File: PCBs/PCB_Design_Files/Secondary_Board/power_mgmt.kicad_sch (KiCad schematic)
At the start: 19 parts, among them Q3 MMBT3904, Q4 MMBT3904, U5 TPS61023DRLR, U6 TLV9101IDCKR

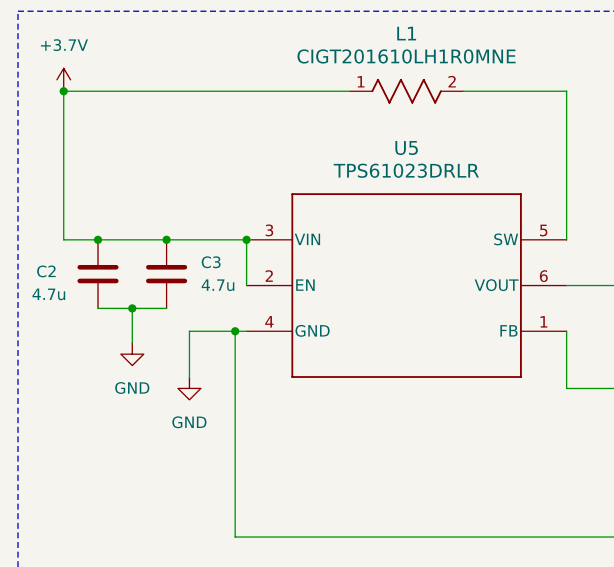
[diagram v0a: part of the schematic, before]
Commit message: updte
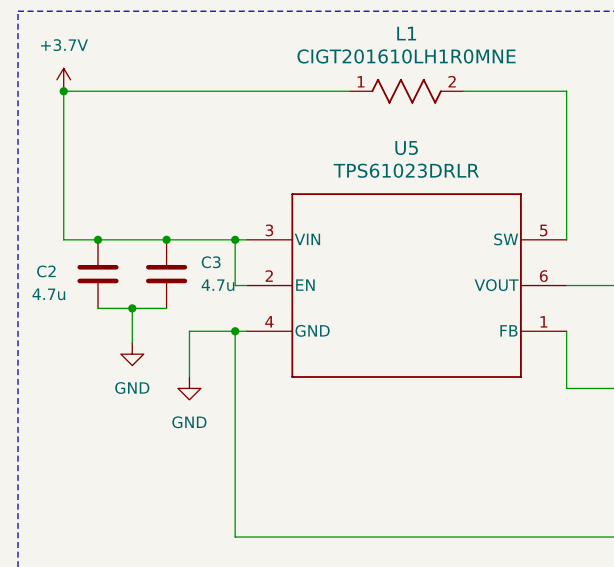
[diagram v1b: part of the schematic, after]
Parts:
- removed U5: TPS61023DRLR, Project Footprints:DRL0006A, symbol TPS61023:TPS61023DRLR
- added U5: TPS61023DRLR, Project Footprints:DRL0006A, symbol Project_Symbols:TPS61023DRLR
- BT1: footprint Diode_THT:D_DO-35_SOD27_P7.62mm_Horizontal -> Connector_JST:JST_PH_S2B-PH-K_1x02_P2.00mm_Horizontal
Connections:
- net +3.7V: now also U5.2 (EN), U5.3 (VIN)
- net +5V: now also U5.6 (VOUT)
- net GND: now also U5.4 (GND)
- net at R1.2, R2.1: now also U5.1 (FB)
- net at L1.2: now also U5.5 (SW)
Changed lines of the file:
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@@
+	)
+	(junction
+		(at 36.83 87.63)
+		(diameter 0)
+		(color 0 0 0 0)
 	)
 	(junction
@@
 	)
 	(junction
-		(at 36.83 87.63)
-		(diameter 0)
-		(color 0 0 0 0)
-	)
-	(junction
 		(at 113.03 82.55)
 		(diameter 0)
@@
 	)
 	(junction
-		(at 38.1 77.47)
-		(diameter 0)
-		(color 0 0 0 0)
-	)
-	(junction
 		(at 91.44 82.55)
 		(diameter 0)
@@
 	)
 	(junction
+		(at 36.83 77.47)
+		(diameter 0)
+		(color 0 0 0 0)
+	)
+	(junction
 		(at 91.44 110.49)
 		(diameter 0)
@@
 	(wire
 		(pts
+			(xy 31.75 87.63) (xy 36.83 87.63)
+		)
+		(stroke
+			(width 0)
+			(type default)
+		)
+	)
+	(wire
+		(pts
 			(xy 157.48 95.25) (xy 144.78 95.25)
 		)
@@
 	(wire
 		(pts
-			(xy 38.1 77.47) (xy 38.1 82.55)
-		)
-		(stroke
-			(width 0)
-			(type default)
-		)
-	)
-	(wire
-		(pts
 			(xy 91.44 92.71) (xy 91.44 93.98)
 		)
@@
 	(wire
 		(pts
-			(xy 38.1 87.63) (xy 36.83 87.63)
-		)
-		(stroke
-			(width 0)
-			(type default)
-		)
-	)
-	(wire
-		(pts
 			(xy 25.4 85.09) (xy 25.4 88.9)
 		)
@@
 	(wire
 		(pts
+			(xy 36.83 77.47) (xy 38.1 77.47)
+		)
+		(stroke
+			(width 0)
+			(type default)
+		)
+	)
+	(wire
+		(pts
 			(xy 144.78 95.25) (xy 144.78 99.06)
 		)
@@
 	(wire
 		(pts
+			(xy 29.21 77.47) (xy 36.83 77.47)
+		)
+		(stroke
+			(width 0)
+			(type default)
+		)
+	)
+	(wire
+		(pts
 			(xy 229.87 99.06) (xy 229.87 80.01)
 		)
@@
 	(wire
 		(pts
-			(xy 36.83 87.63) (xy 31.75 87.63)
-		)
-		(stroke
-			(width 0)
-			(type default)
-		)
-	)
-	(wire
-		(pts
 			(xy 91.44 93.98) (xy 91.44 96.52)
 		)
@@
 	(wire
 		(pts
+			(xy 38.1 82.55) (xy 36.83 82.55)
+		)
+		(stroke
+			(width 0)
+			(type default)
+		)
+	)
+	(wire
+		(pts
 			(xy 49.53 60.96) (xy 17.78 60.96)
 		)
@@
 	(wire
 		(pts
-			(xy 29.21 77.47) (xy 38.1 77.47)
+			(xy 36.83 87.63) (xy 38.1 87.63)
 		)
 		(stroke
@@
 		(pts
 			(xy 254 134.62) (xy 254 130.81)
+		)
+		(stroke
+			(width 0)
+			(type default)
+		)
+	)
+	(wire
+		(pts
+			(xy 36.83 77.47) (xy 36.83 82.55)
 		)
 		(stroke
@@
 	)
 	(symbol
-		(lib_id "TPS61023:TPS61023DRLR")
-		(at 55.88 82.55 0)
-		(unit 1)
-		(exclude_from_sim no)
-		(in_bom yes)
-		(on_board no)
-		(dnp no)
-		(fields_autoplaced yes)
-		(property "Reference" "U5"
-			(at 55.88 67.31 0)
-			(effects
-				(font
-					(size 1.524 1.524)
-				)
-			)
-		)
-		(property "Value" "TPS61023DRLR"
-			(at 55.88 69.85 0)
-			(effects
-				(font
-					(size 1.524 1.524)
-				)
-			)
-		)
-		(property "Footprint" "Project Footprints:DRL0006A"
-			(at 55.88 82.55 0)
-			(effects
-				(font
-					(size 1.27 1.27)
-					(italic yes)
-				)
-				(hide yes)
-			)
-		)
-		(property "Datasheet" "https://www.ti.com/lit/gpn/tps61023"
-			(at 55.88 82.55 0)
-			(effects
-				(font
-					(size 1.27 1.27)
-					(italic yes)
-				)
-				(hide yes)
-			)
-		)
-		(property "Description" ""
-			(at 55.88 82.55 0)
-			(effects
-				(font
-					(size 1.27 1.27)
-				)
-				(hide yes)
-			)
-		)
-		(pin "1"
-		)
-		(pin "6"
-		)
-		(pin "3"
-		)
-		(pin "4"
-		)
-		(pin "5"
-		)
-		(pin "2"
-		)
-		(instances
-			(project "Secondary_Board"
-				(path "/2f5986e4-77b2-4f5d-ab91-80ba6228eb8b/3db8306c-5846-4ae5-ba17-fe529edf9e71"
-					(reference "U5")
-					(unit 1)
-				)
-			)
-			(project "power_mgmt"
-				(path "/c7abdc65-9966-45f8-babc-768b62a50249"
-					(reference "U1")
-					(unit 1)
-				)
-			)
-		)
-	)
-	(symbol
 		(lib_id "power:PWR_FLAG")
 		(at 36.83 26.67 0)
@@
 	)
 	(symbol
+		(lib_id "Project_Symbols:TPS61023DRLR")
+		(at 55.88 82.55 0)
+		(unit 1)
+		(exclude_from_sim no)
+		(in_bom yes)
+		(on_board yes)
+		(dnp no)
+		(fields_autoplaced yes)
+		(property "Reference" "U5"
+			(at 55.88 67.31 0)
+			(effects
+				(font
+					(size 1.524 1.524)
+				)
+			)
+		)
+		(property "Value" "TPS61023DRLR"
+			(at 55.88 69.85 0)
+			(effects
+				(font
+					(size 1.524 1.524)
+				)
+			)
+		)
+		(property "Footprint" "Project Footprints:DRL0006A"
+			(at 55.372 95.25 0)
+			(effects
+				(font
+					(size 1.27 1.27)
+					(italic yes)
+				)
+				(hide yes)
+			)
+		)
+		(property "Datasheet" "https://www.ti.com/lit/gpn/tps61023"
+			(at 57.15 93.472 0)
+			(effects
+				(font
+					(size 1.27 1.27)
+					(italic yes)
+				)
+				(hide yes)
+			)
+		)
+		(property "Description" ""
+			(at 55.88 82.55 0)
+			(effects
+				(font
+					(size 1.27 1.27)
+				)
+				(hide yes)
+			)
+		)
+		(pin "5"
+		)
+		(pin "6"
+		)
+		(pin "1"
+		)
+		(pin "3"
+		)
+		(pin "2"
+		)
+		(pin "4"
+		)
+		(instances
+			(project ""
+				(path "/2f5986e4-77b2-4f5d-ab91-80ba6228eb8b/3db8306c-5846-4ae5-ba17-fe529edf9e71"
+					(reference "U5")
+					(unit 1)
+				)
+			)
+		)
+	)
+	(symbol
 		(lib_id "Device:C")
 		(at 21.59 81.28 0)
@@
 			)
 		)
-		(property "Footprint" "Diode_THT:D_DO-35_SOD27_P7.62mm_Horizontal"
+		(property "Footprint" "Connector_JST:JST_PH_S2B-PH-K_1x02_P2.00mm_Horizontal"
 			(at 27.94 32.766 90)
 			(effects
